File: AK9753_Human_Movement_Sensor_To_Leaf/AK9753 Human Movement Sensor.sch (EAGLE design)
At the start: 12 parts, among them U2 AK9753

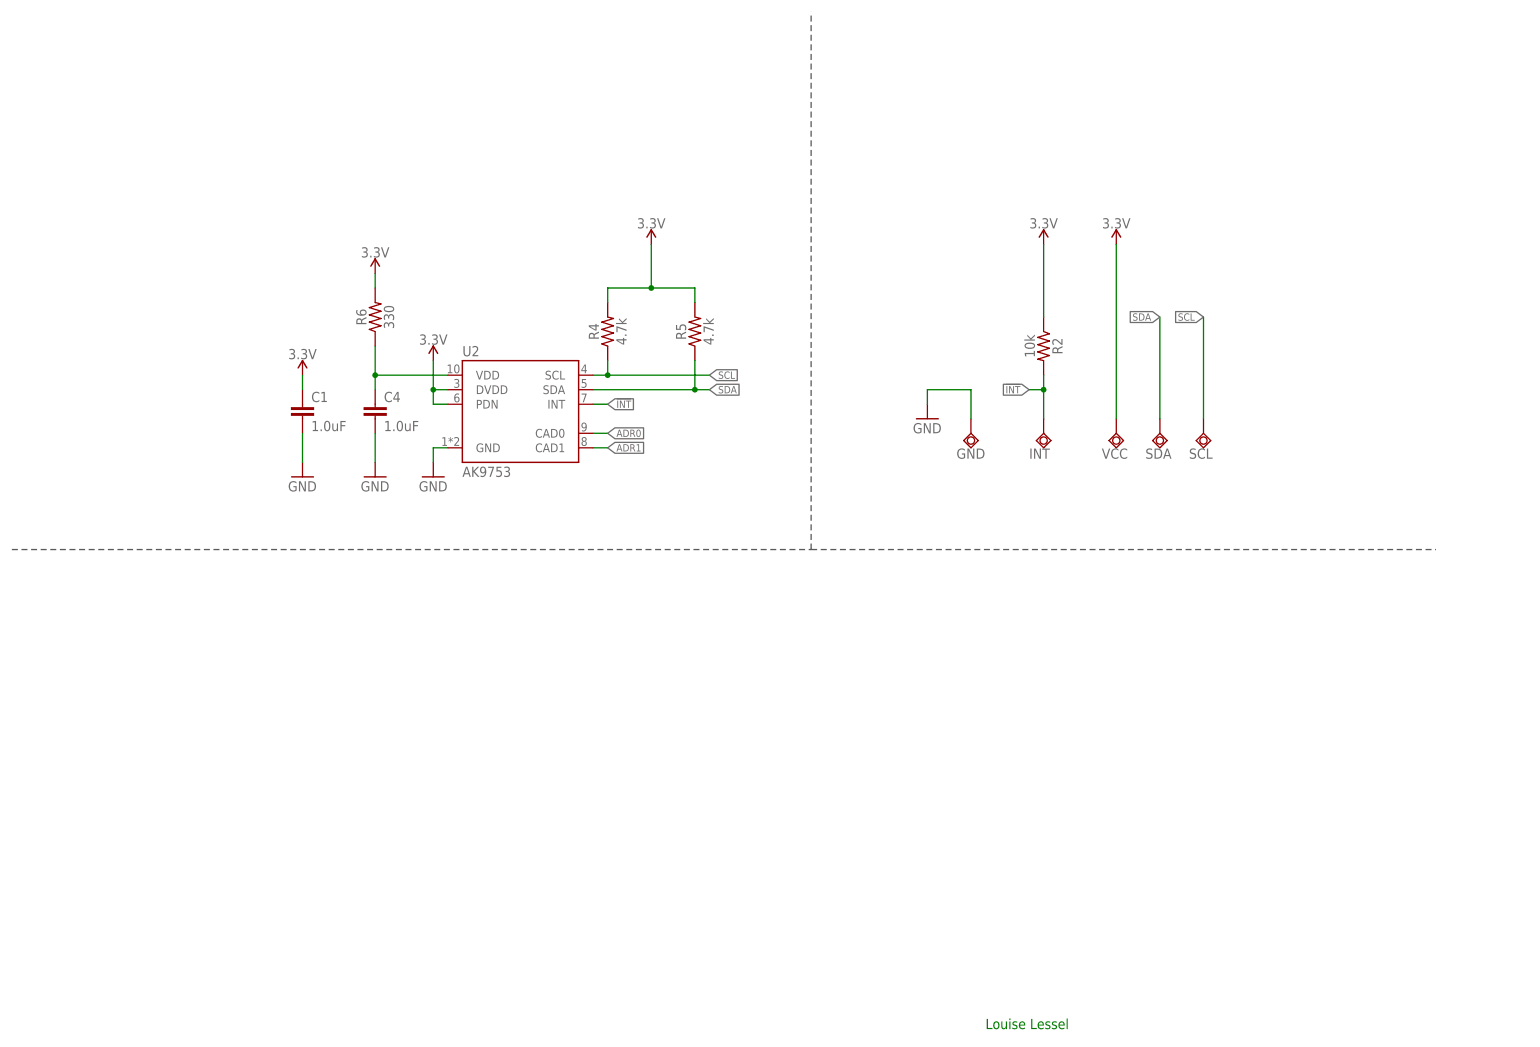
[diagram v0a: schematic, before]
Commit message: PDFs
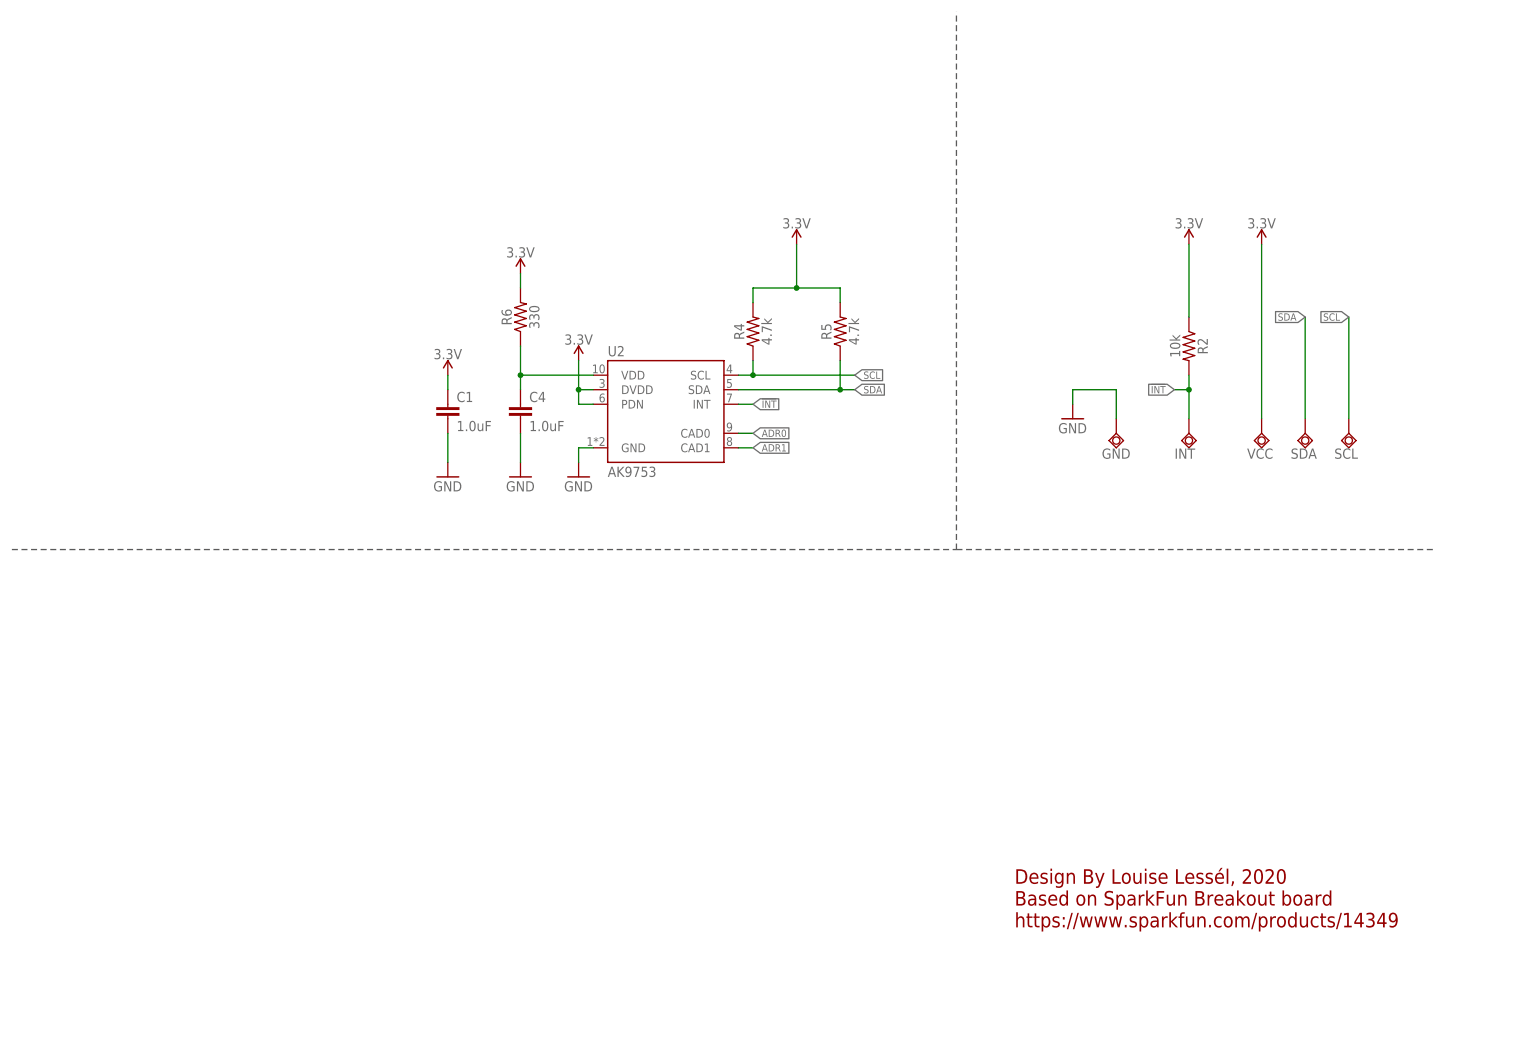
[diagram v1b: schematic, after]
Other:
- note added: "Design By Louise Lessél, 2020 Based on SparkFun Breakout board https://www.sparkfun.com/products/14349"
- note removed: "Louise Lessel"
- moved on the sheet: C1, C4, GND, INT, R2, R4, R5, R6, SCL, SDA, U2, VCC
